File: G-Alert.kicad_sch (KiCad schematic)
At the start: 16 parts, among them P1 USB_C_Plug_USB2.0, SW1 SW_Push, U1 MQ-4b, U2 LM393

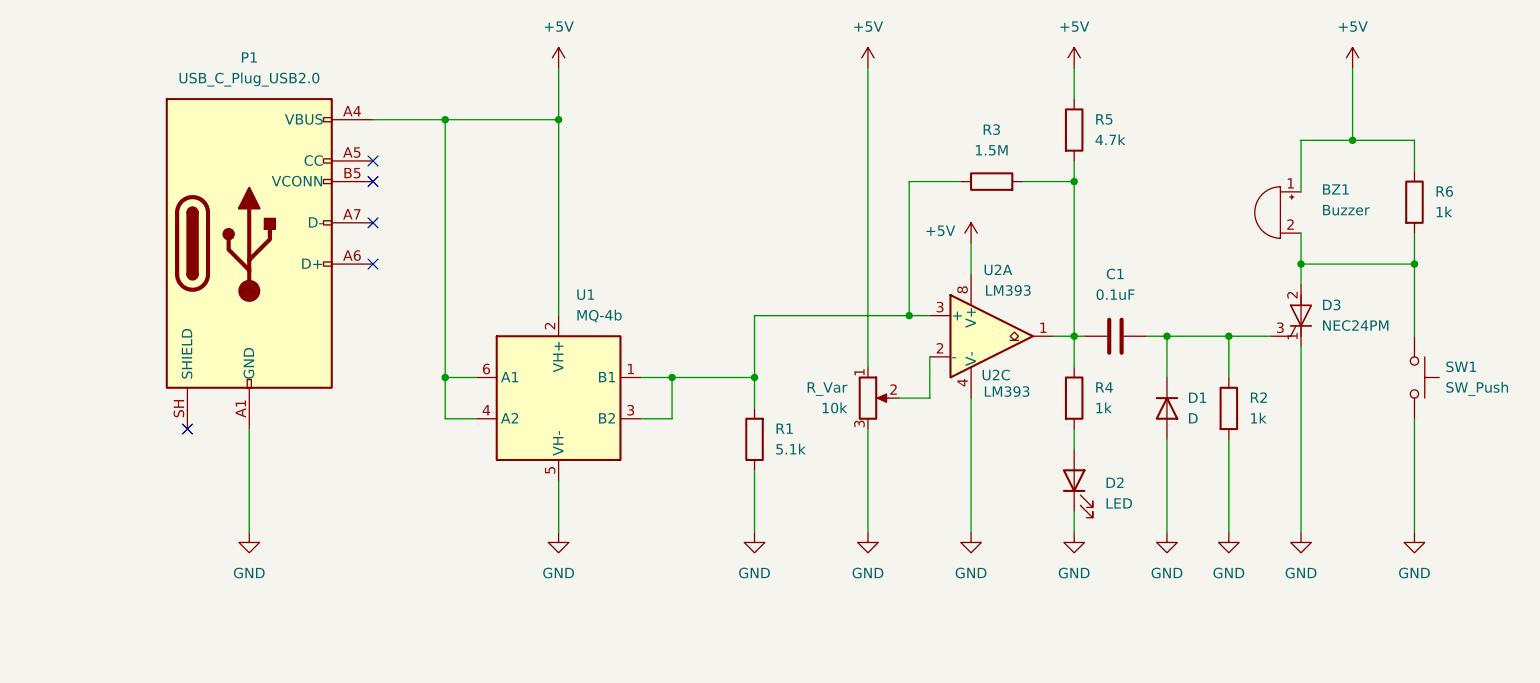
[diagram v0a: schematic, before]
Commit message: Final Update on Schematics
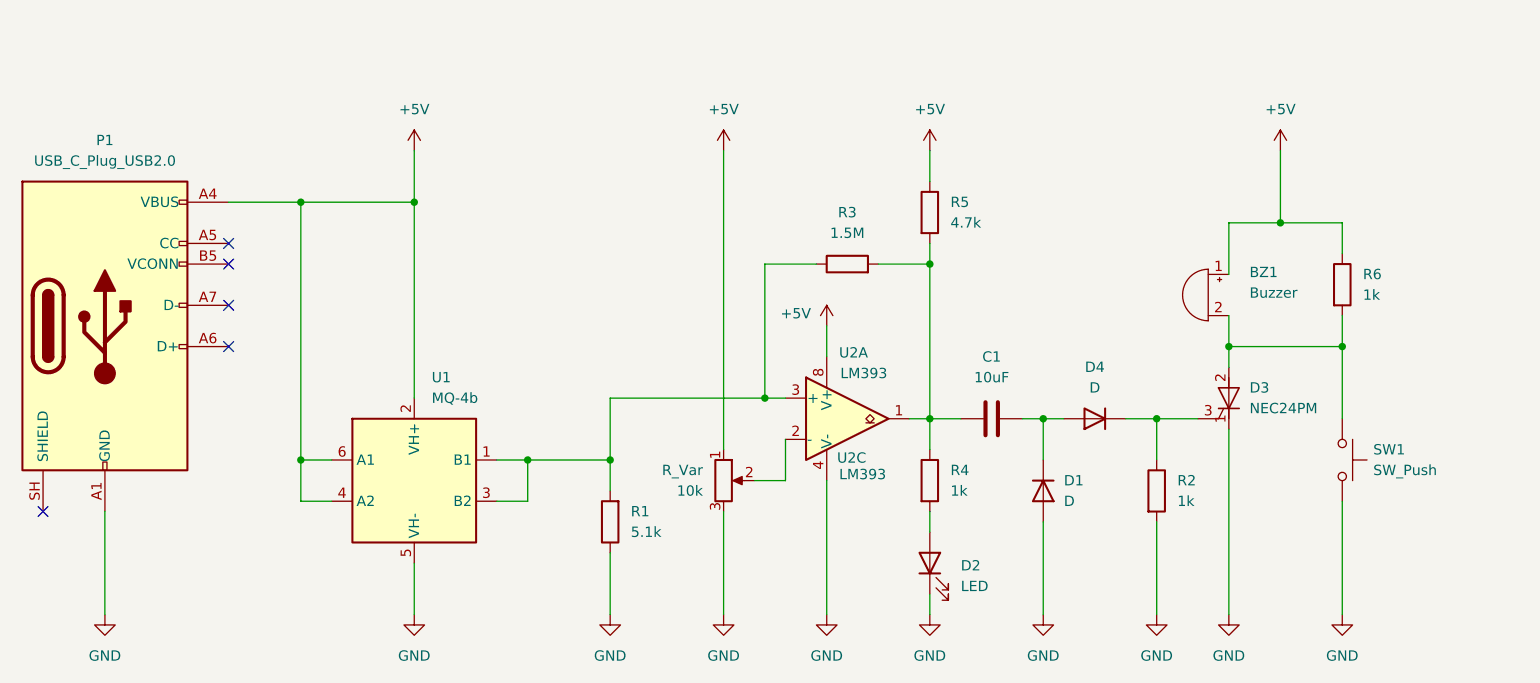
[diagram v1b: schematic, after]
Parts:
- added D4: D, symbol Device:D
- C1: value 0.1uF -> 10uF
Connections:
- net at D3.3 (G), R2.1: now also D4.1 (K); no longer C1.2, D1.1 (K)
- new net: C1.2, D1.1 (K), D4.2 (A)
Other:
- moved on the sheet: BZ1, D1, D2, D3, P1, R1, R2, R3, R4, R5, R6, R_Var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
